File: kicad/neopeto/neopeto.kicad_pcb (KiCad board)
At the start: 2 copper layers, 168.9 x 76.2 mm, 148 parts, among them J1 Conn_01x10_Pin, J2 Conn_01x10_Pin, J3 Conn_01x10_Pin, J4 PJ-307, J5 Conn_01x10, J6 Conn_01x10, J7 Conn_01x10, U1 74HC00, U10 74HC590, U11 74HC590, U12 74HC590, U13 74HC245, U14 K6X4008C1F, U15 74HC245, U16 74HC245, U17 LM358LV, U18 LM358LV, U19 LM358LV, U2 74LVC1G00, U20 Pico, U21 TLC7258C, U22 TLC7258C, U23 74HC4017, U24 74HC86, U25 74AUP1G08, U26 74LVC1G332, U27 74LVC1G332, U3 CH32V003JxMx, U4 82C55A_PLCC, U5 82C54_PLCC, U6 74LS139, U7 74HC245, U8 74HC245, U9 74HC245, X1 ECS-2520MV-12MHZ

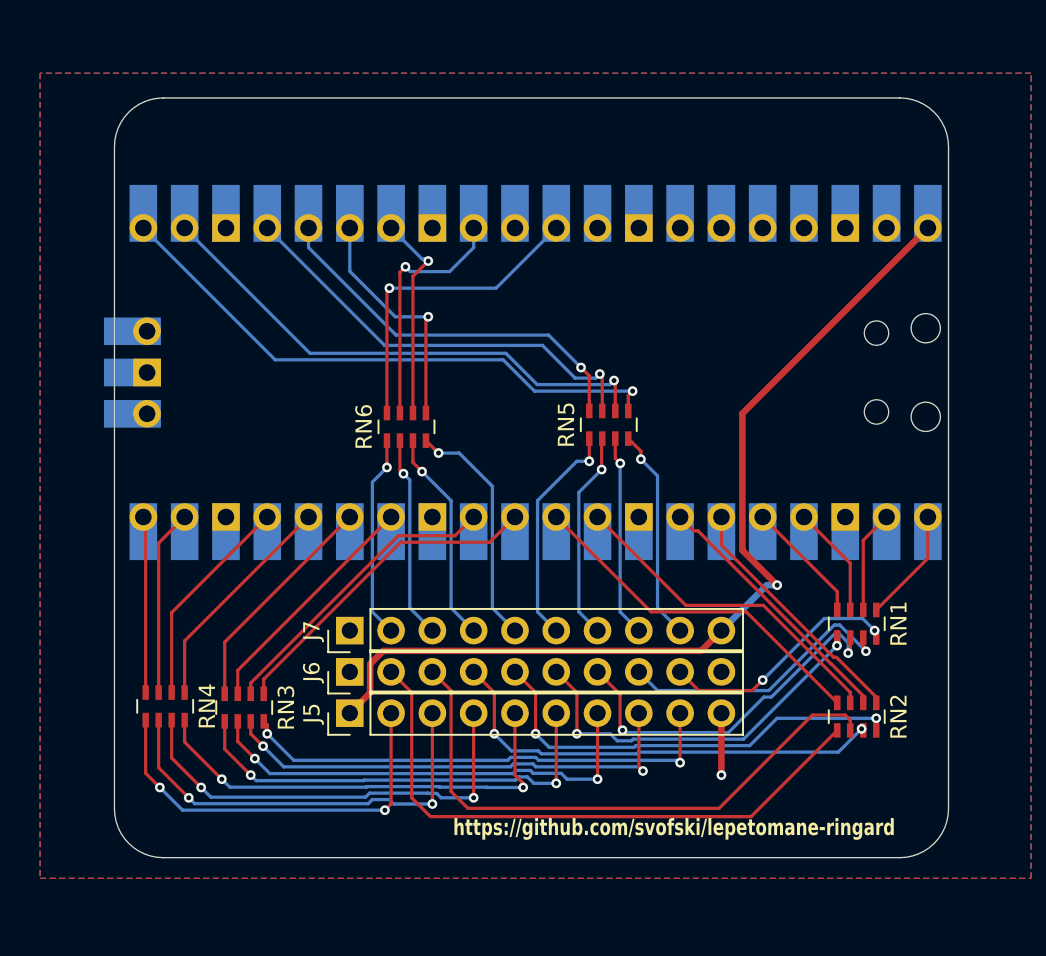
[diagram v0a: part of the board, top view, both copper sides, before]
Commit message: before separation
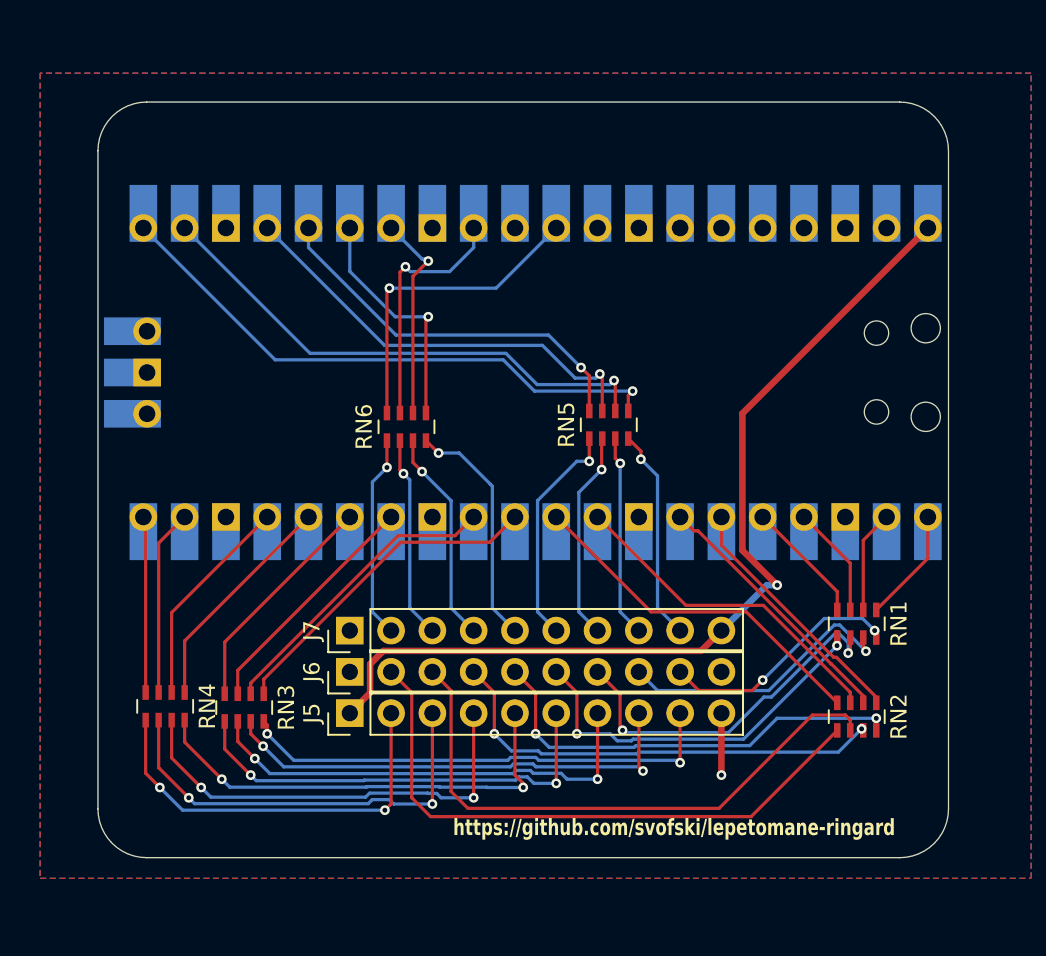
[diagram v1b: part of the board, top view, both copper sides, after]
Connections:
- net Net-(RN1-R1.1) renamed /PI_GPIO0
- net Net-(RN1-R2.1) renamed /PI_GPIO1
- net Net-(RN1-R3.1) renamed /PI_GPIO2
- net Net-(RN1-R4.1) renamed /PI_GPIO3
- net Net-(RN2-R1.1) renamed /PI_GPIO4
- net Net-(RN2-R2.1) renamed /PI_GPIO5
- net Net-(RN2-R3.1) renamed /PI_GPIO6
- net Net-(RN2-R4.1) renamed /PI_GPIO7
- net Net-(RN3-R1.1) renamed /PI_GPIO8
- net Net-(RN3-R2.1) renamed /PI_GPIO9
- net Net-(RN3-R3.1) renamed /PI_GPIO10
- net Net-(RN3-R4.1) renamed /PI_GPIO11
- net Net-(RN4-R1.1) renamed /PI_GPIO12
- net Net-(RN4-R2.1) renamed /PI_GPIO13
- net Net-(RN4-R3.1) renamed /PI_GPIO14
- net Net-(RN4-R4.1) renamed /PI_GPIO15
- net Net-(RN5-R1.2) renamed /PI_GPIO19
- net Net-(RN5-R2.2) renamed /PI_GPIO18
- net Net-(RN5-R3.2) renamed /PI_GPIO17
- net Net-(RN5-R4.2) renamed /PI_GPIO16
- net Net-(RN6-R1.2) renamed /PI_GPIO26
- net Net-(RN6-R2.2) renamed /PI_GPIO22
- net Net-(RN6-R3.2) renamed /PI_GPIO21
- net Net-(RN6-R4.2) renamed /PI_GPIO20
- U20 pad 36: unconnected-(U20-3V3-Pad36) -> /PI_3V3
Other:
- outline, holes or cut-outs redrawn
